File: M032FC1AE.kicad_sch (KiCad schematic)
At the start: 35 parts, among them IC1 M032FC1AE, J1 Conn_01x10, J2 Conn_01x03, J4 USB_C_Receptacle_USB2.0_16P, J5 Conn_01x03, J6 Conn_01x05, J7 Conn_02x08_Odd_Even, Q1 S8050, SW1 SW_Push, SW2 SW_Push, U1 AMS1117-1.8, U2 AMS1117-3.3, U3 USBLC6-2SC6

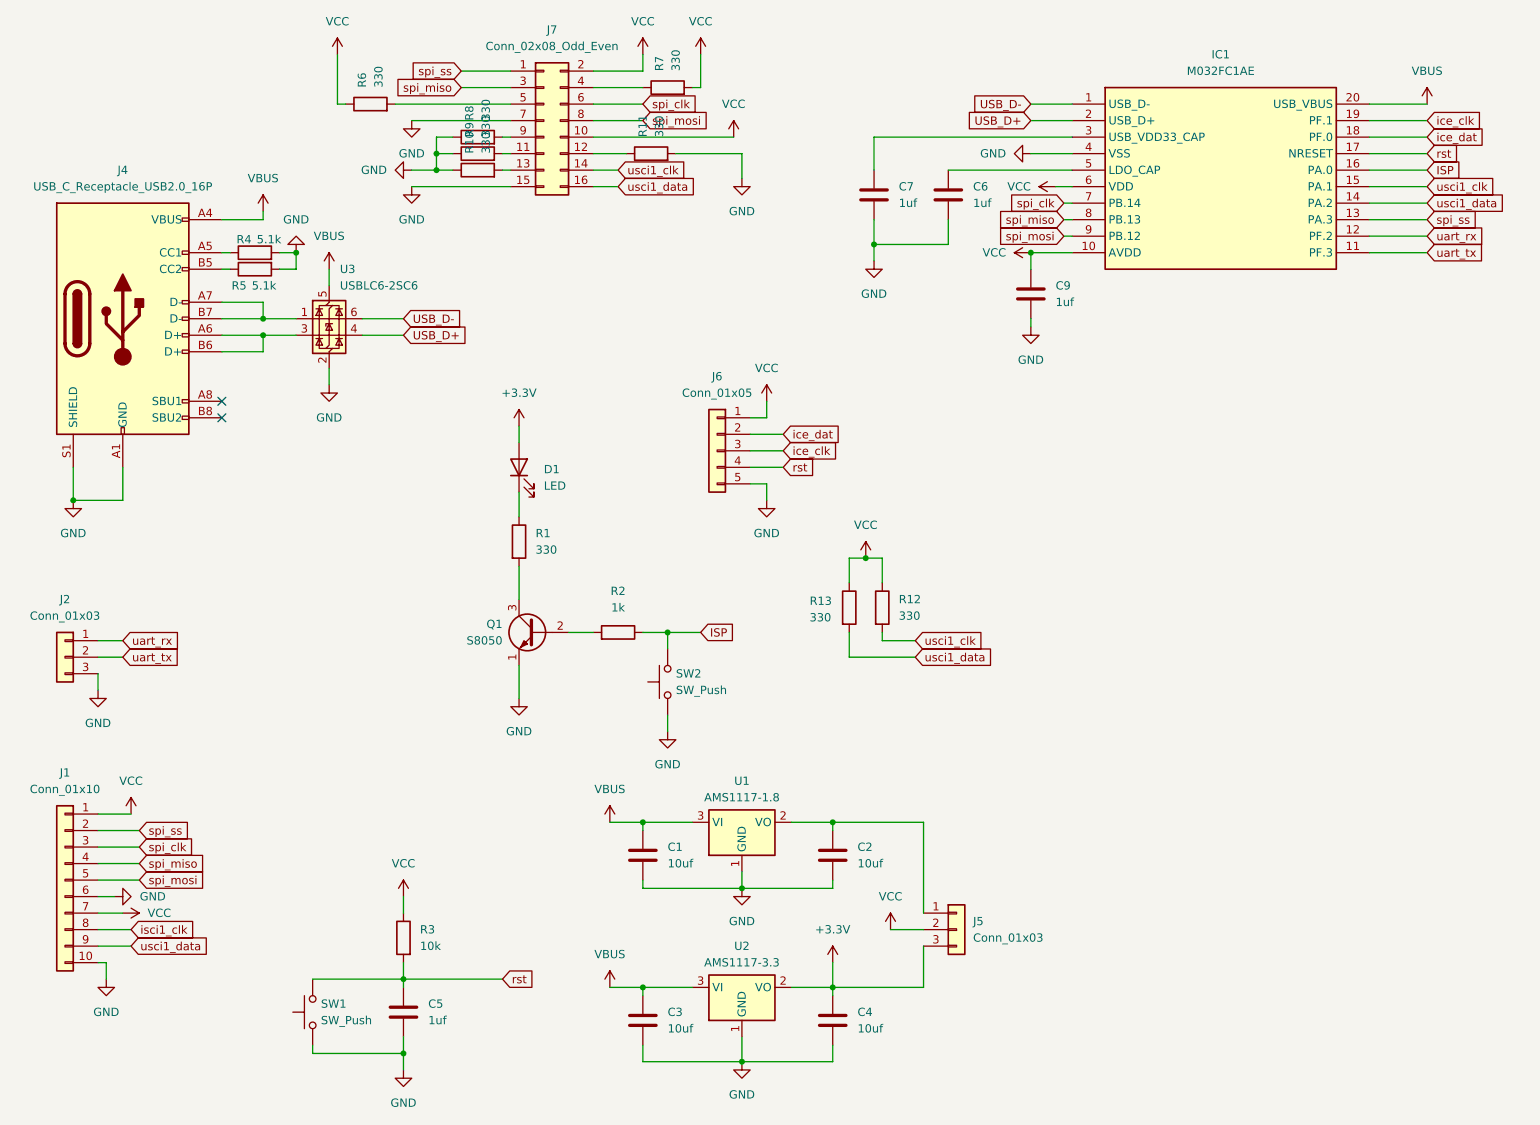
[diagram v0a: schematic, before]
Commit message: ffffddd
Change-Id: I1eeee01593b08b9acbec1eab3a106692ce76c6c6
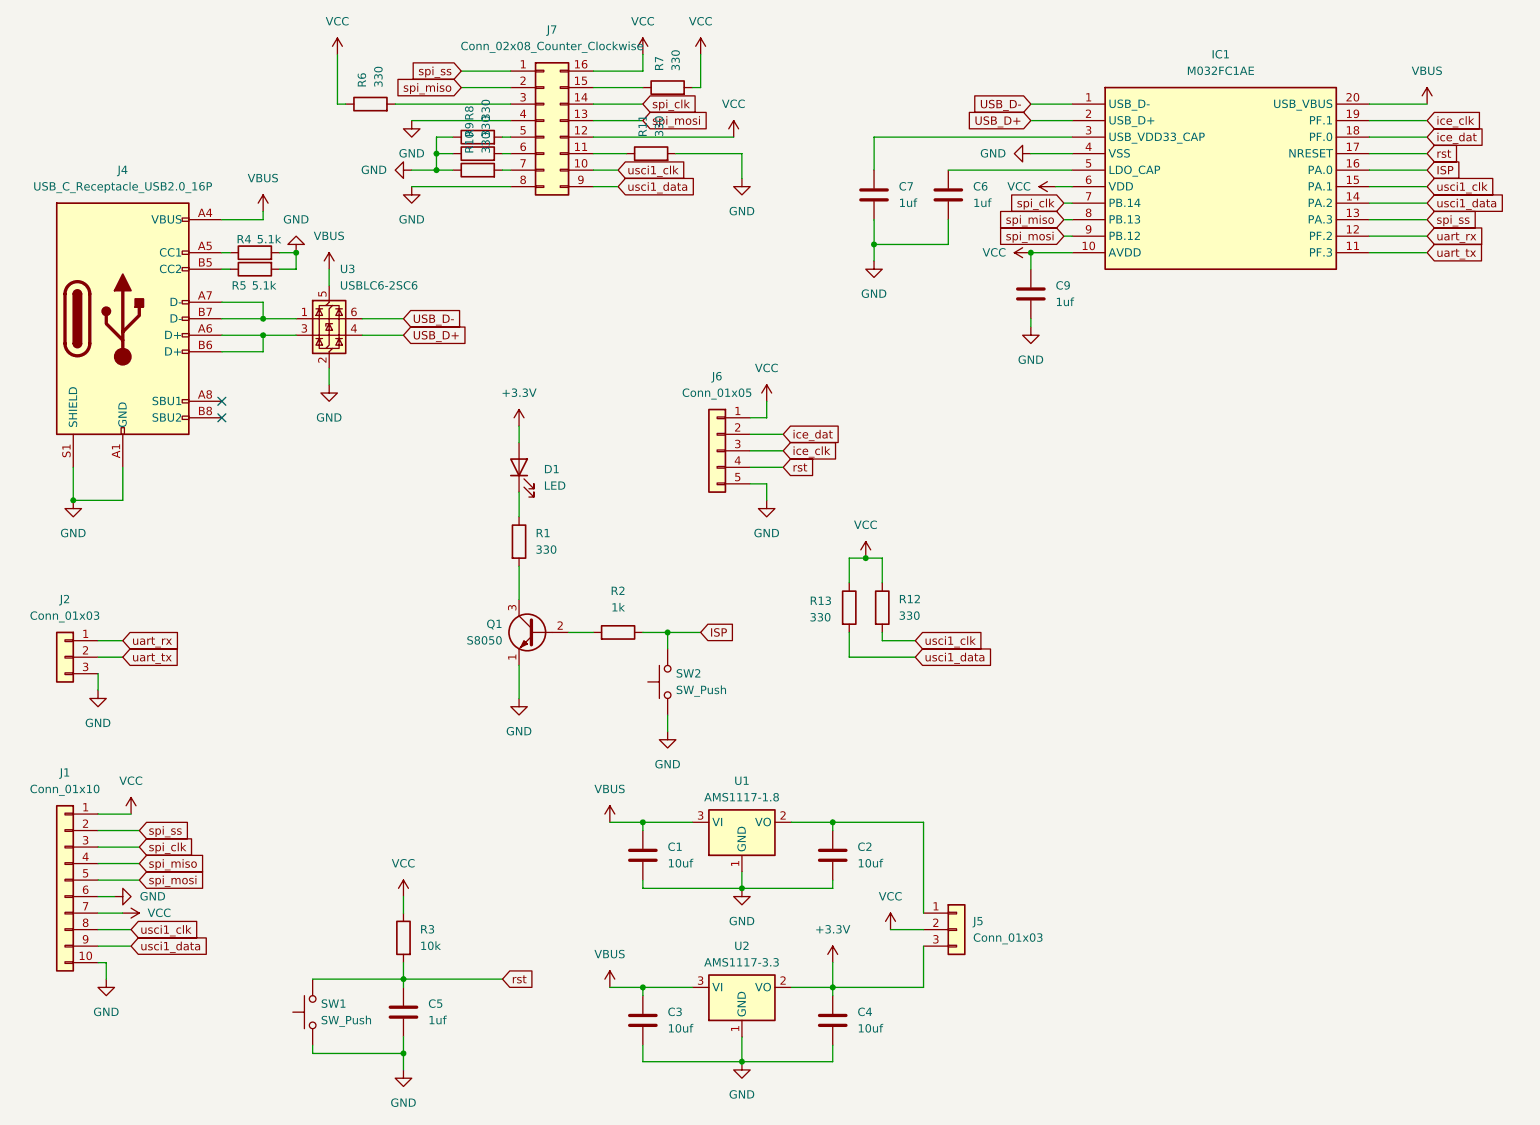
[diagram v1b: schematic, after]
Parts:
- removed J7: Conn_02x08_Odd_Even, Socket:DIP_Socket-16_W4.3_W5.08_W7.62_W10.16_W10.9_3M_216-3340-00-0602J, symbol Connector_Generic:Conn_02x08_Odd_Even
- added J7: Conn_02x08_Counter_Clockwise, Socket:DIP_Socket-16_W4.3_W5.08_W7.62_W10.16_W10.9_3M_216-3340-00-0602J, symbol Connector_Generic:Conn_02x08_Counter_Clockwise
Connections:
- net isci1_clk is gone; now on net usci1_clk: J1.8 (Pin_8)
- net GND: now also J7.4 (Pin_4), J7.8 (Pin_8)
- net VCC: now also J7.12 (Pin_12), J7.16 (Pin_16)
- net spi_clk: now also J7.14 (Pin_14)
- net spi_miso: now also J7.2 (Pin_2)
- net spi_mosi: now also J7.13 (Pin_13)
- net spi_ss: now also J7.1 (Pin_1)
- net usci1_clk: now also J7.10 (Pin_10)
- net usci1_data: now also J7.9 (Pin_9)
- net at R11.1: now also J7.11 (Pin_11)
- net at R9.2: now also J7.6 (Pin_6)
- net at R10.2: now also J7.7 (Pin_7)
- net at R7.1: now also J7.15 (Pin_15)
- net at R6.2: now also J7.3 (Pin_3)
- net at R8.2: now also J7.5 (Pin_5)

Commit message: dfdfdfdf
Change-Id: I4bedd6ca326a9b17d3d6f978c0846dd558e38f70
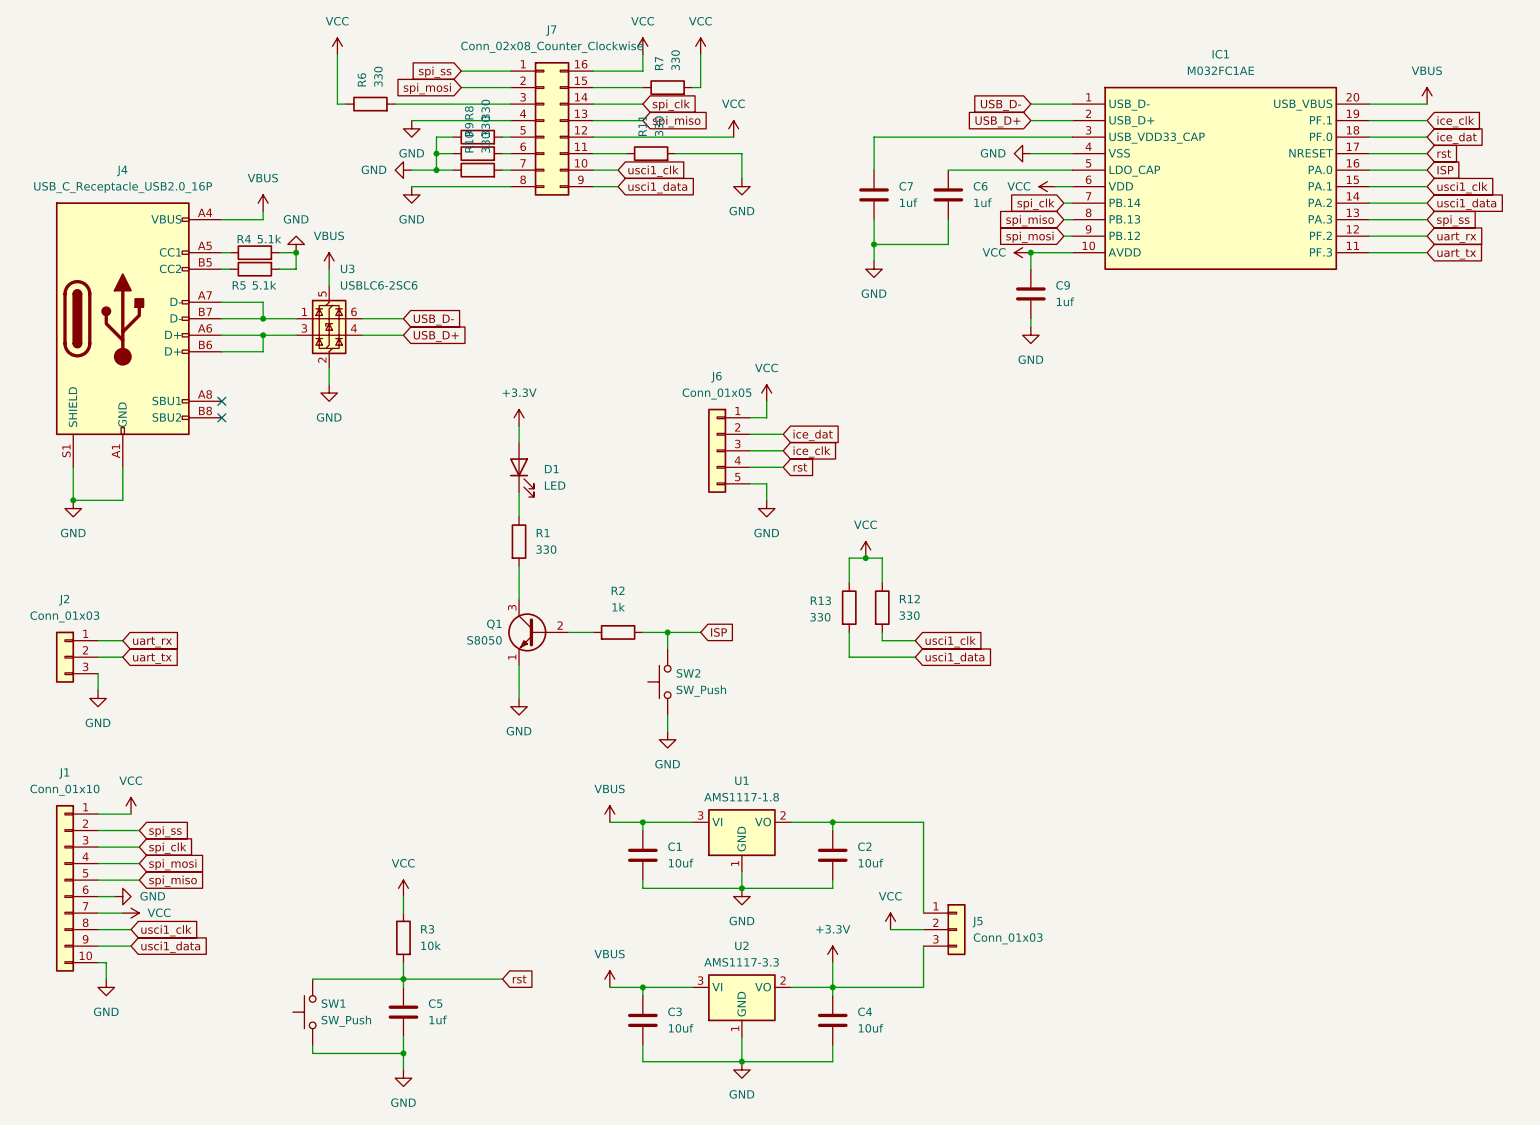
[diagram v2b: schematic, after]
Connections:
- net spi_miso: now also J1.5 (Pin_5), J7.13 (Pin_13); no longer J1.4 (Pin_4), J7.2 (Pin_2)
- net spi_mosi: now also J1.4 (Pin_4), J7.2 (Pin_2); no longer J1.5 (Pin_5), J7.13 (Pin_13)

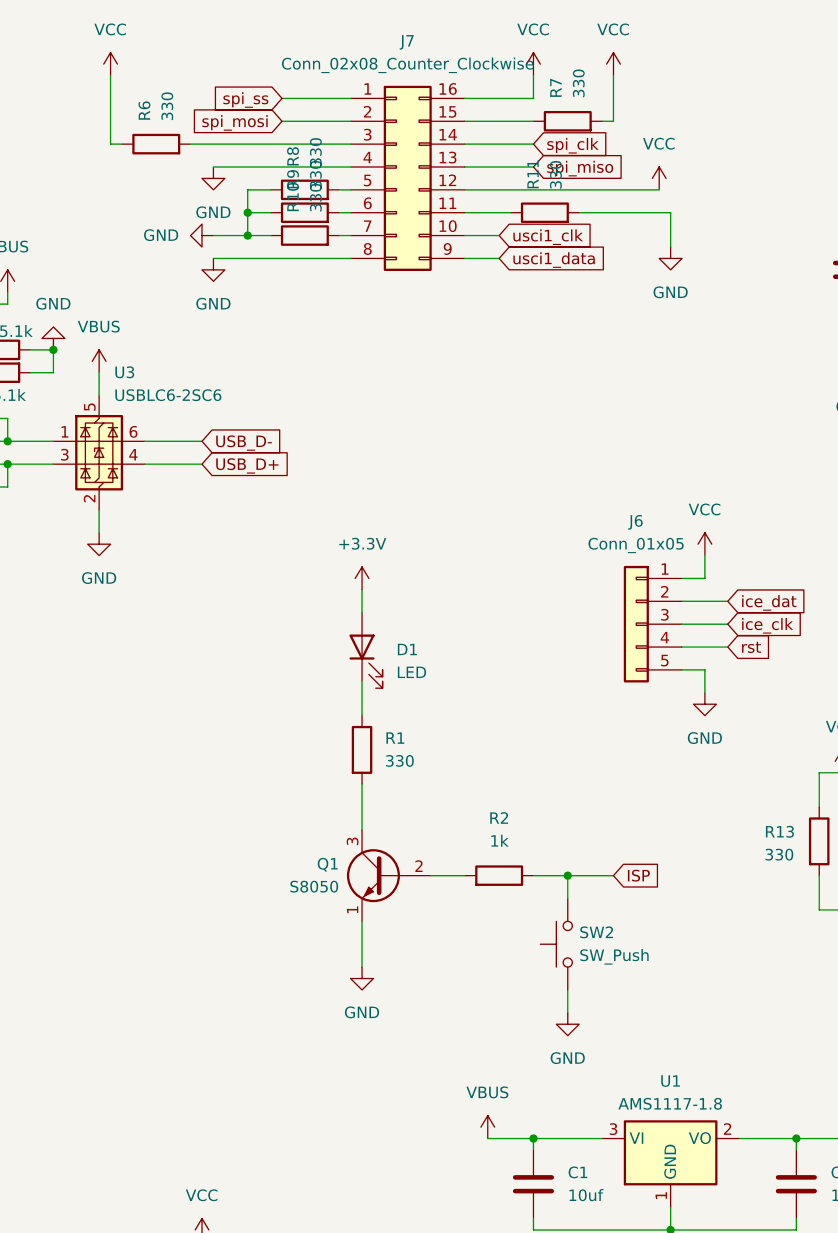
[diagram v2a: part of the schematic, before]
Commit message: lalala
Change-Id: I877491cc6b06ae896878915a1c7d8004ea38277d
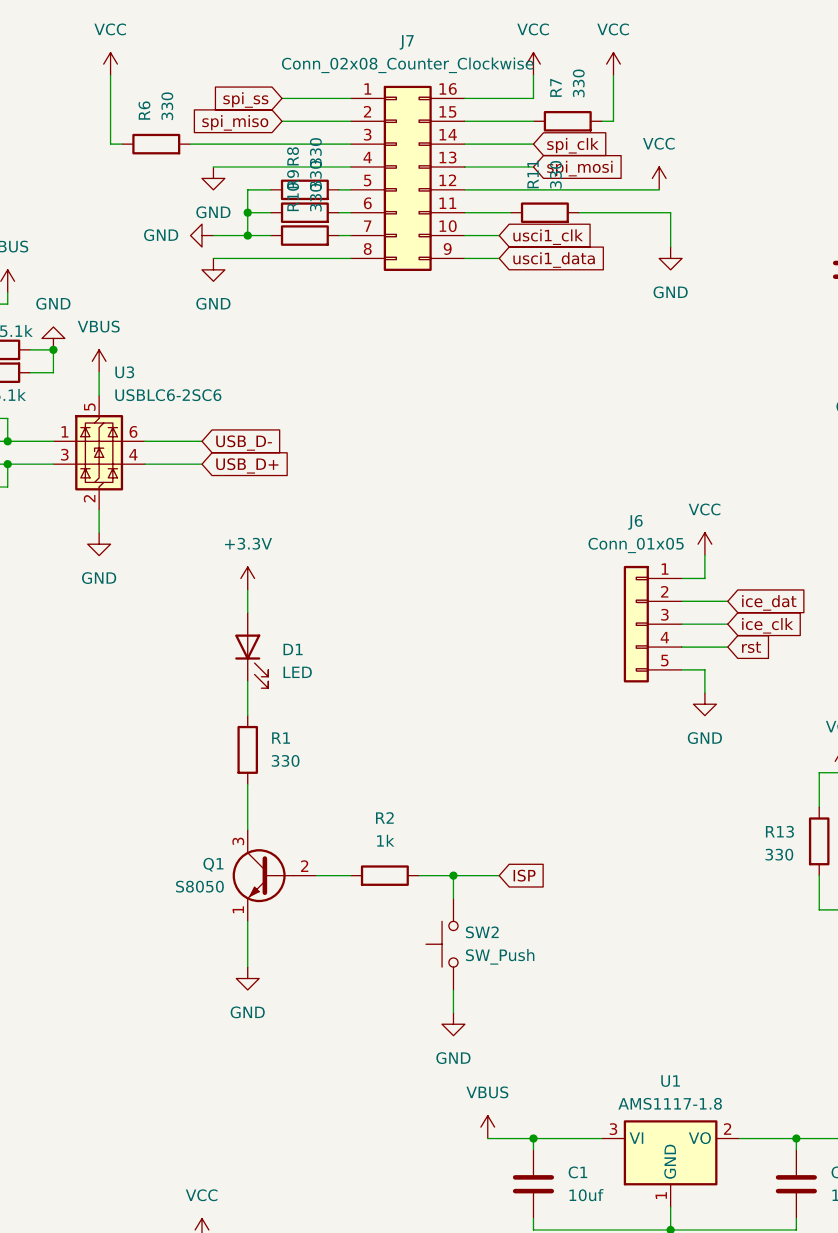
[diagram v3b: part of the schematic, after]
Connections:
- net spi_miso: now also J7.2 (Pin_2); no longer J7.13 (Pin_13)
- net spi_mosi: now also J7.13 (Pin_13); no longer J7.2 (Pin_2)
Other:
- moved on the sheet: D1, Q1, R1, R2, SW2
